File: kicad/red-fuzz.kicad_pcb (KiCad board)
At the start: 2 copper layers, 59 x 90 mm, 67 parts, among them J1 2.1mm Center Neg Insulated, J2 Input Stereo, J3 TEST_1P, J4 TEST_1P, J5 TEST_1P, J6 Output Mono, Q1 j201, SW1 SW_3PDT, SW2 SW_SPDT, U1 NE5532

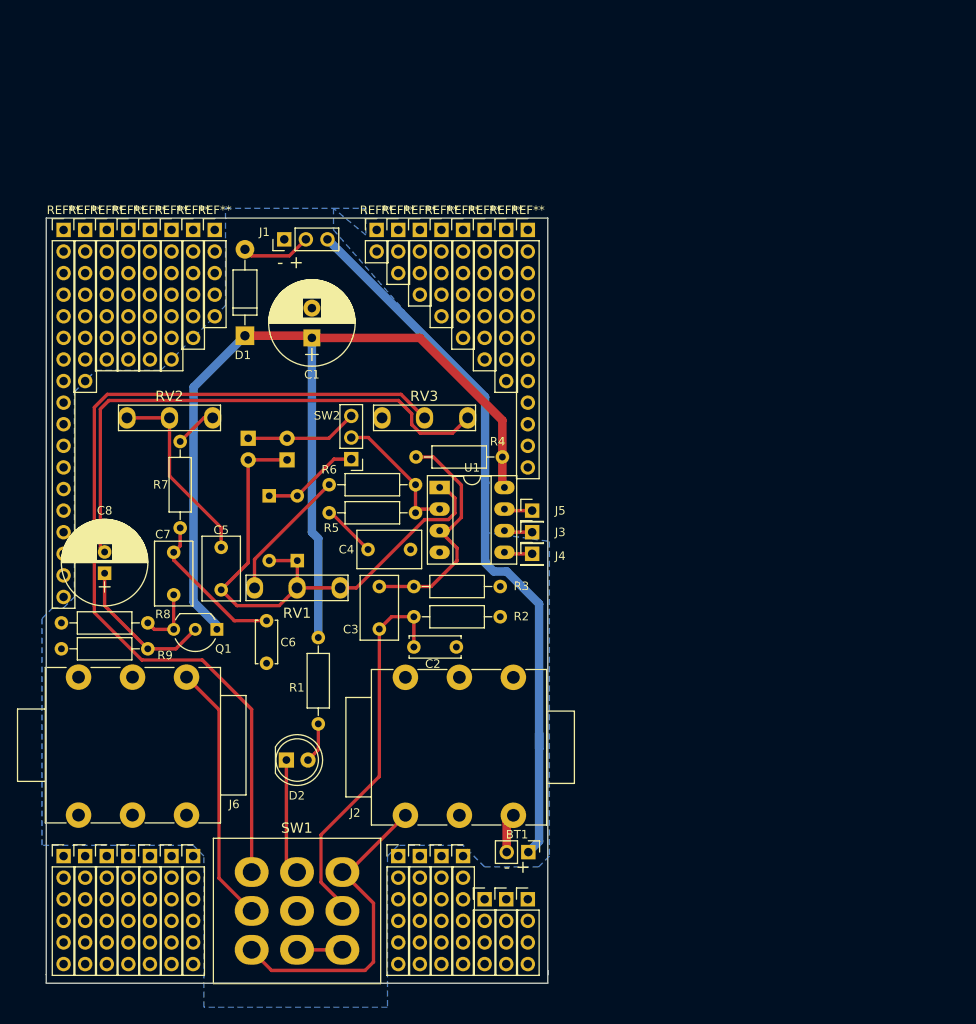
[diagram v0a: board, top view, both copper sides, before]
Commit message: Project Rev. B
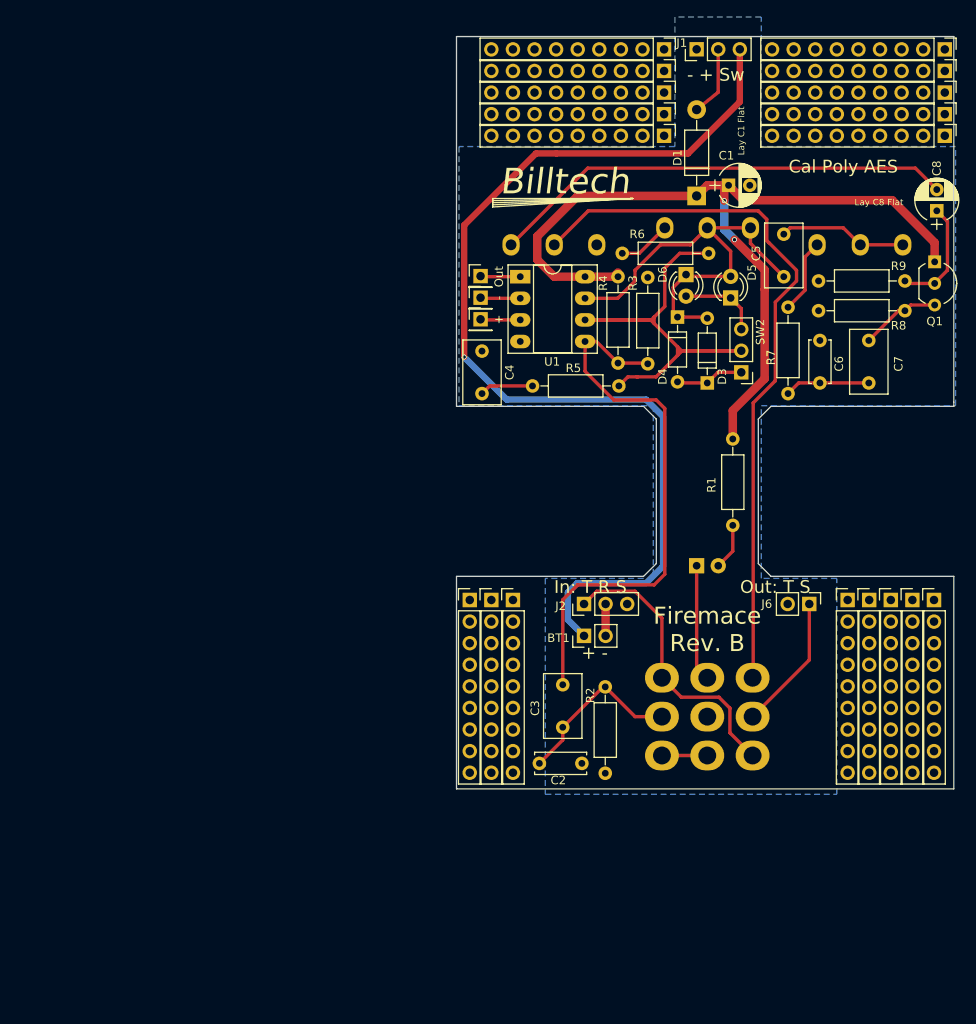
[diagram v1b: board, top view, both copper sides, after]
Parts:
- removed ? (x11): , Pin_Headers:Pin_Header_Straight_1x06_Pitch2.54mm
- removed ? (x3): , Pin_Headers:Pin_Header_Straight_1x04_Pitch2.54mm
- removed the REF** at (90.6, 74.9)
- removed the REF** at (132.5, 74.9)
- removed the REF** at (130.0, 74.9)
- removed the REF** at (127.5, 74.9)
- removed the REF** at (124.9, 74.9)
- removed the REF** at (122.4, 74.9)
- removed the REF** at (85.5, 74.9)
- removed the REF** at (88.1, 74.9)
- removed the REF** at (93.2, 74.9)
- removed the REF** at (95.7, 74.9)
- removed the REF** at (98.2, 74.9)
- removed the REF** at (100.8, 74.9)
- removed the REF** at (103.3, 74.9)
- removed the REF** at (140.2, 74.9)
- removed the REF** at (137.6, 74.9)
- removed the REF** at (135.1, 74.9)
- added REF**: Pin_Header_Straight_1x09_Pitch2.54mm, Pin_Headers:Pin_Header_Straight_1x09_Pitch2.54mm, F.Cu at (189.2, 63.8)
- added REF**: Pin_Header_Straight_1x09_Pitch2.54mm, Pin_Headers:Pin_Header_Straight_1x09_Pitch2.54mm, F.Cu at (135.9, 118.4)
- added REF**: Pin_Header_Straight_1x09_Pitch2.54mm, Pin_Headers:Pin_Header_Straight_1x09_Pitch2.54mm, F.Cu at (185.4, 118.4)
- added REF**: Pin_Header_Straight_1x09_Pitch2.54mm, Pin_Headers:Pin_Header_Straight_1x09_Pitch2.54mm, F.Cu at (180.3, 118.4)
- added REF**: Pin_Header_Straight_1x09_Pitch2.54mm, Pin_Headers:Pin_Header_Straight_1x09_Pitch2.54mm, F.Cu at (177.8, 118.4)
- added REF**: Pin_Header_Straight_1x09_Pitch2.54mm, Pin_Headers:Pin_Header_Straight_1x09_Pitch2.54mm, F.Cu at (182.8, 118.4)
- added REF**: Pin_Header_Straight_1x09_Pitch2.54mm, Pin_Headers:Pin_Header_Straight_1x09_Pitch2.54mm, F.Cu at (187.9, 118.4)
- added REF**: Pin_Header_Straight_1x09_Pitch2.54mm, Pin_Headers:Pin_Header_Straight_1x09_Pitch2.54mm, F.Cu at (133.3, 118.4)
- added REF**: Pin_Header_Straight_1x09_Pitch2.54mm, Pin_Headers:Pin_Header_Straight_1x09_Pitch2.54mm, F.Cu at (138.4, 118.4)
- added REF**: Pin_Header_Straight_1x09_Pitch2.54mm, Pin_Headers:Pin_Header_Straight_1x09_Pitch2.54mm, F.Cu at (156.2, 53.7)
- added REF**: Billtech, feetprints:Billtech, F.Cu at (145.3, 69.4)
- added REF**: Pin_Header_Straight_1x09_Pitch2.54mm, Pin_Headers:Pin_Header_Straight_1x09_Pitch2.54mm, F.Cu at (189.2, 61.3)
- added REF**: Pin_Header_Straight_1x09_Pitch2.54mm, Pin_Headers:Pin_Header_Straight_1x09_Pitch2.54mm, F.Cu at (189.2, 58.7)
- added REF**: Pin_Header_Straight_1x09_Pitch2.54mm, Pin_Headers:Pin_Header_Straight_1x09_Pitch2.54mm, F.Cu at (189.2, 56.2)
- added REF**: Pin_Header_Straight_1x09_Pitch2.54mm, Pin_Headers:Pin_Header_Straight_1x09_Pitch2.54mm, F.Cu at (189.2, 53.7)
- added REF**: Pin_Header_Straight_1x09_Pitch2.54mm, Pin_Headers:Pin_Header_Straight_1x09_Pitch2.54mm, F.Cu at (156.2, 63.8)
- added REF**: Pin_Header_Straight_1x09_Pitch2.54mm, Pin_Headers:Pin_Header_Straight_1x09_Pitch2.54mm, F.Cu at (156.2, 61.3)
- added REF**: Pin_Header_Straight_1x09_Pitch2.54mm, Pin_Headers:Pin_Header_Straight_1x09_Pitch2.54mm, F.Cu at (156.2, 58.7)
- added REF**: Pin_Header_Straight_1x09_Pitch2.54mm, Pin_Headers:Pin_Header_Straight_1x09_Pitch2.54mm, F.Cu at (156.2, 56.2)
- C1: footprint Capacitors_THT:CP_Radial_D10.0mm_P3.50mm -> Capacitors_THT:CP_Radial_D5.0mm_P2.50mm
- C8: footprint Capacitors_THT:CP_Radial_D10.0mm_P2.50mm -> Capacitors_THT:CP_Radial_D5.0mm_P2.50mm
- D2, SW1: moved to B.Cu
- D3, D4, D5, D6: moved to F.Cu
- J2: footprint Connectors:NMJ6HCD2 -> Pin_Headers:Pin_Header_Straight_1x03_Pitch2.54mm
- J6: footprint Connectors:NMJ6HCD2 -> Pin_Headers:Pin_Header_Straight_1x02_Pitch2.54mm
- RV1: footprint guitar-projects:pot_16mm_long_lead -> pot_16mm_long_lead; moved to B.Cu
- RV2: footprint pot_16mm_long_lead -> feetprints:pot_16mm_long_lead; moved to B.Cu
- RV3: footprint guitar-projects:pot_16mm_long_lead -> feetprints:pot_16mm_long_lead; moved to B.Cu
- moved C8 106.8 mm to (188.3, 72.6)
- moved R9 99.0 mm to (184.5, 80.9)
- moved R8 96.3 mm to (184.5, 84.4)
- moved Q1 94.9 mm to (188.0, 78.6), turned to 270 degrees
- moved C7 87.1 mm to (180.3, 87.9), turned to 270 degrees
- moved RV2 83.8 mm to (179.3, 76.6), turned to 180 degrees
- moved C5 75.7 mm to (170.3, 75.4)
- moved J6 73.8 mm to (173.3, 118.9)
- moved R7 73.2 mm to (170.8, 94.1)
- moved C6 70.8 mm to (174.5, 92.9), turned to 90 degrees
- moved RV1 64.2 mm to (161.3, 74.6)
- moved D5 59.1 mm to (164.0, 82.9), turned to 90 degrees
- moved D1 55.6 mm to (160.0, 70.9)
- moved R1 54.1 mm to (164.3, 109.6)
- moved J1 53.4 mm to (160.0, 53.6)
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- renumbered J4 to +, J3 to -, J5 to Out
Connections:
- U1 pad 1: Net-(C5-Pad2) -> Net-(J5-Pad1)
- U1 pad 2: Net-(R5-Pad1) -> Net-(J3-Pad1)
- U1 pad 3: Net-(C3-Pad1) -> Net-(J4-Pad1)
- U1 pad 5: Net-(J4-Pad1) -> Net-(C3-Pad1)
- U1 pad 6: Net-(J3-Pad1) -> Net-(R5-Pad1)
- U1 pad 7: Net-(J5-Pad1) -> Net-(C5-Pad2)
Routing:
- net Net-(R5-Pad1): track 16.2 -> 58.2 mm
- net Net-(C3-Pad1): track 28.5 -> 65.9 mm
- net /Batt+: track 85.6 -> 122.4 mm, vias 0 -> 1
- net Net-(C2-Pad1): track 45.3 -> 20.5 mm
- net Net-(RV3-Pad2): track 107.1 -> 84.5 mm
- net +9V: track 116.1 -> 101.1 mm, vias 0 -> 2
- net Net-(J6-Pad1): track 30.7 -> 16.0 mm
- net Net-(C5-Pad2): track 64.5 -> 52.7 mm
- net Net-(R6-Pad1): track 15.8 -> 6.24 mm
- net Net-(C8-Pad2): track 63.7 -> 54.9 mm
- net Net-(C6-Pad1): track 18.0 -> 10.0 mm
- net Net-(C5-Pad1): track 22.7 -> 15.1 mm
- net Net-(C8-Pad1): track 17.5 -> 13.6 mm
- net Net-(J2-Pad1): track 38.1 -> 34.3 mm
- net Net-(R7-Pad2): track 4.98 -> 8.76 mm
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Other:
- board size 59 x 90 mm -> 58.5 x 88.5 mm
- net class +9V: clearance 0.2 -> 0.3; trace_width 1 -> 0.75
- net class Default: clearance 0.2 -> 0.3
- rule trace_clearance: 0.2 -> 0.3
- board text added: "- + Sw"
- board text added: "Cal Poly AES"
- board text added: "Firemace Rev. B"
- board text added: "In: T R S"
- board text added: "Lay C1 Flat"
- board text added: "Lay C8 Flat"
- board text added: "Out: T S"
- board text added: "Pin 1"
- board text removed: "- +"
